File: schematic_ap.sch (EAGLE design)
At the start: 36 parts, among them M1 WIRELESS-NRF24L01, U1 ATMEGA328P_TQFP, U3 MPU-6050

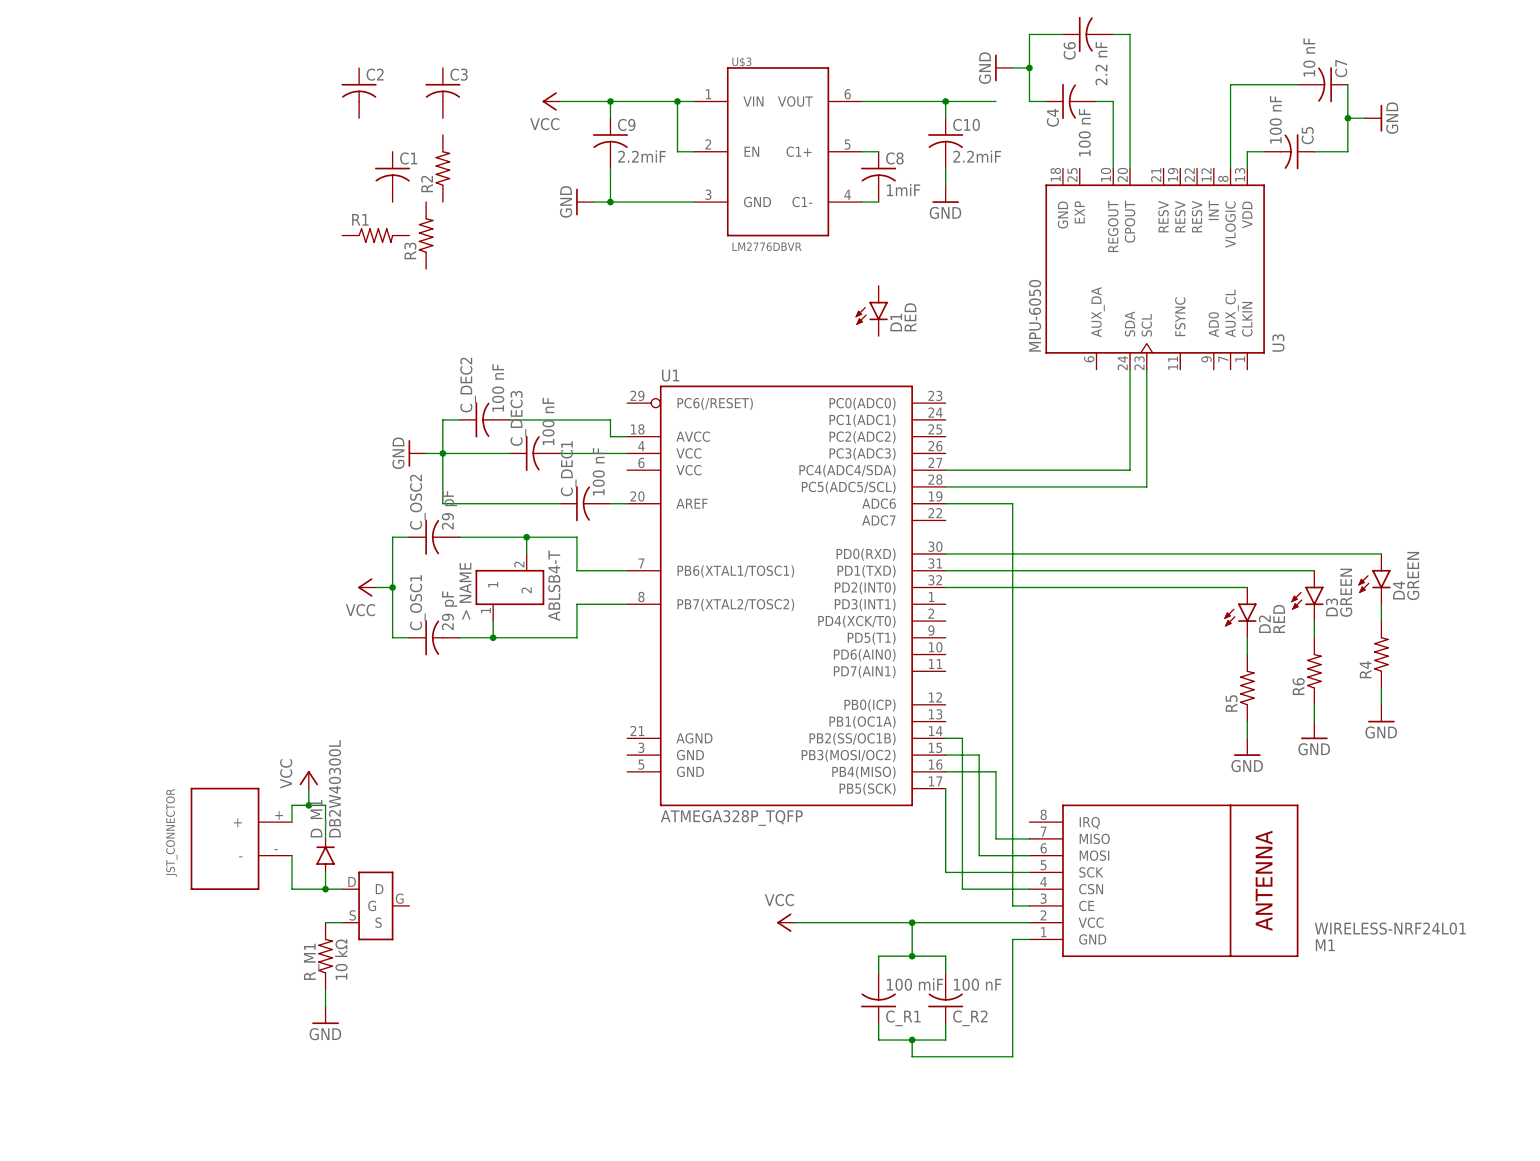
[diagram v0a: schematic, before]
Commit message: Schematic Wiring
Wiring of parts
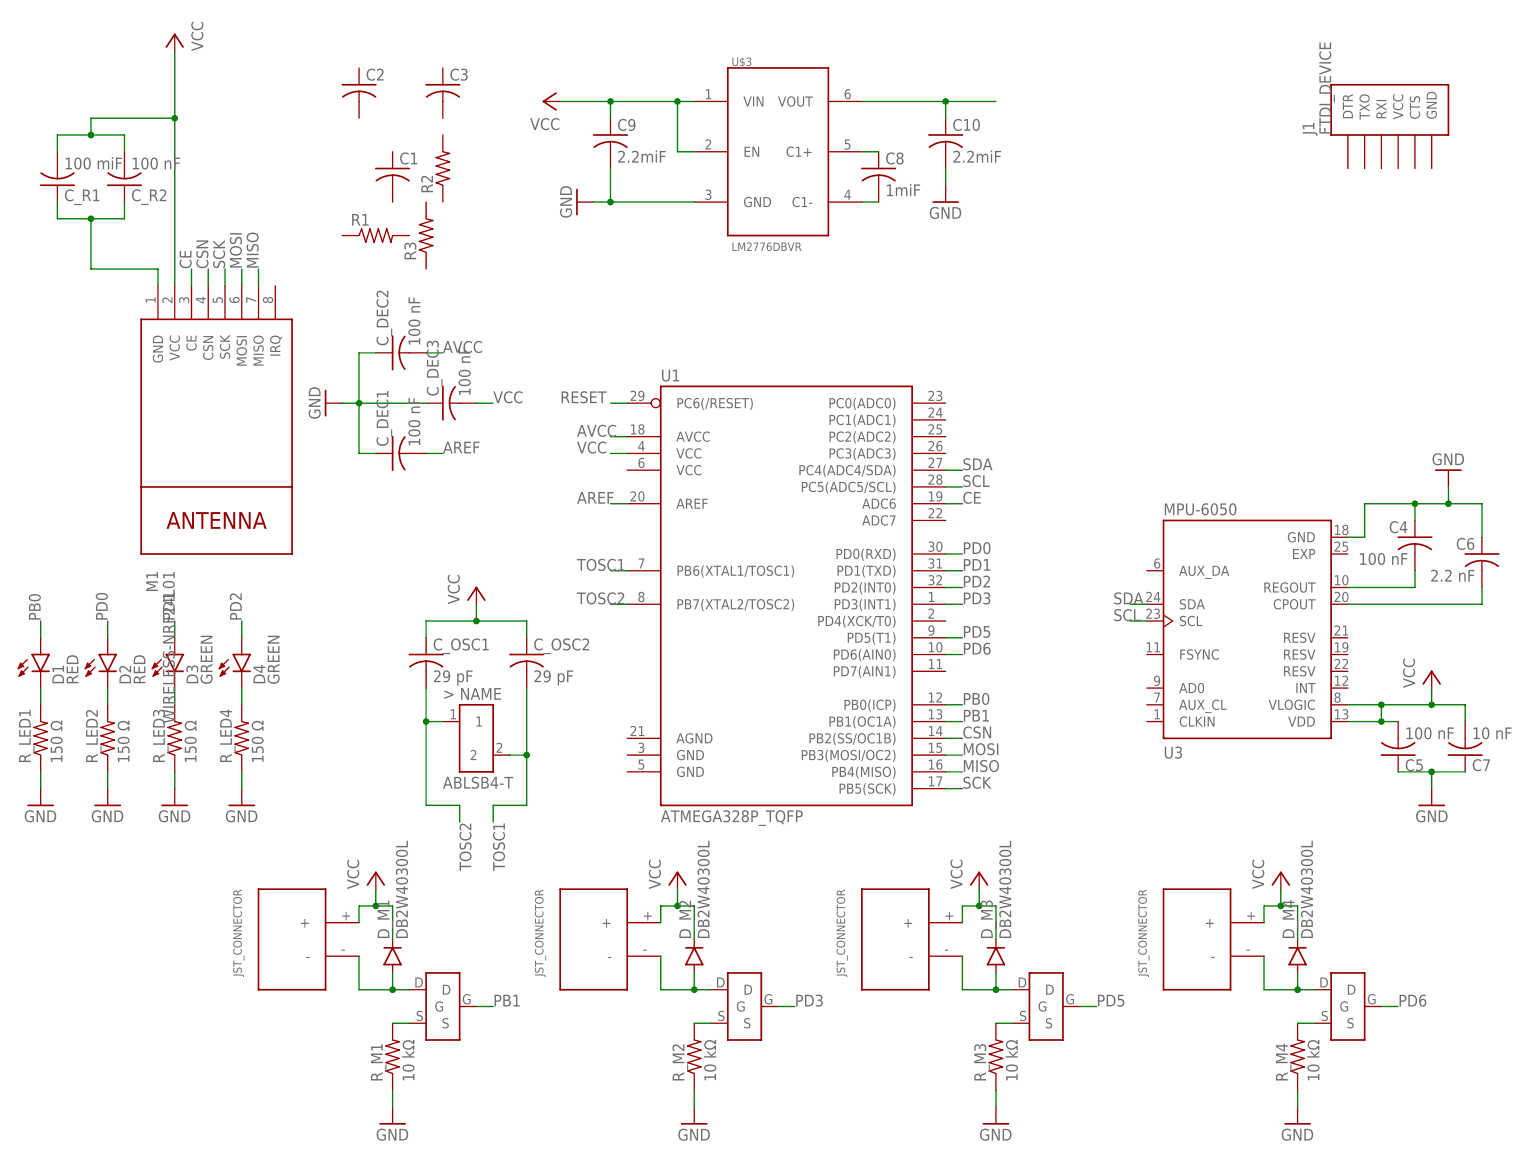
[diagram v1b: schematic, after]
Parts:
- removed R4, R5, R6: (no value), resistor:R-US_R0603
- added D_M2, D_M3, D_M4: DB2W40300L, quad:DB2W40300L
- added J1: FTDI_DEVICE, quad:FTDI_DEVICE
- added R_LED1, R_LED2, R_LED3, R_LED4: 150 Ω, resistor:R-US_R0603
- added R_M2, R_M3, R_M4: 10 kΩ, resistor:R-US_R0603
- added U$1, U$6, U$8: 2N7002P, 2N7002P:2N7002P
- added U$5, U$7, U$9: JST_CONNECTOR_FEMALE, quad:JST_CONNECTOR_FEMALE
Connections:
- net N$1 renamed AVCC
- net N$10 renamed TOSC2
- net N$16 renamed SCL
- net N$17 renamed SDA
- net N$22 renamed PD1
- net N$24 renamed CSN
- net N$25 renamed MOSI
- net N$26 renamed MISO
- net N$27 renamed SCK
- net N$29 renamed CE
- net N$4 renamed AREF
- net N$9 renamed TOSC1
- removed net N$3: C_DEC3.2, U1.VCC@4
- removed net N$7: C5.2, U3.VDD
- removed net N$8: C7.2, U3.VLOGIC
- new net N$22: R_M3.2, U$6.S
- new net N$24: D_M3.PPIN, U$6.D, U$7.-
- new net N$25: R_M4.2, U$8.S
- new net N$26: D_M4.PPIN, U$8.D, U$9.-
- new net N$30: D1.C, R_LED1.2
- new net PB0: D1.A, U1.PB0(ICP)
- new net PB1: U$2.G, U1.PB1(OC1A)
- new net PD0: D2.A, U1.PD0(RXD)
- new net PD2: D4.A, U1.PD2(INT0)
- new net PD3: U$1.G, U1.PD3(INT1)
- new net PD5: U$6.G, U1.PD5(T1)
- new net PD6: U$8.G, U1.PD6(AIN0)
- new net RESET: U1.PC6(/RESET)
- net GND: now also R_LED1.1, R_LED2.1, R_LED3.1, R_LED4.1, R_M2.1, R_M3.1, R_M4.1, U3.GND; no longer R4.1, R5.1, R6.1
- net N$18: now also R_M2.2, U$1.S; no longer D4.A, U1.PD0(RXD)
- net N$19: now also R_LED4.2; no longer R4.2
- net N$20: now also D_M2.PPIN, U$1.D, U$5.-; no longer D2.A, U1.PD2(INT0)
- net N$21: now also R_LED2.2; no longer R5.2
- net N$23: now also R_LED3.2; no longer R6.2
- net VCC: now also C5.2, C7.2, C_DEC3.2, D_M2.GPIN, D_M3.GPIN, D_M4.GPIN, U$5.+, U$7.+, U$9.+, U1.VCC@4, U3.VDD, U3.VLOGIC
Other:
- moved on the sheet: C4, C5, C6, C7, C_DEC1, C_DEC2, C_DEC3, C_OSC1, C_OSC2, C_R1, C_R2, D1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
